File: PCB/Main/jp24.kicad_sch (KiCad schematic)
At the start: 1 part, among them U1 ORANGE_PI_CM4

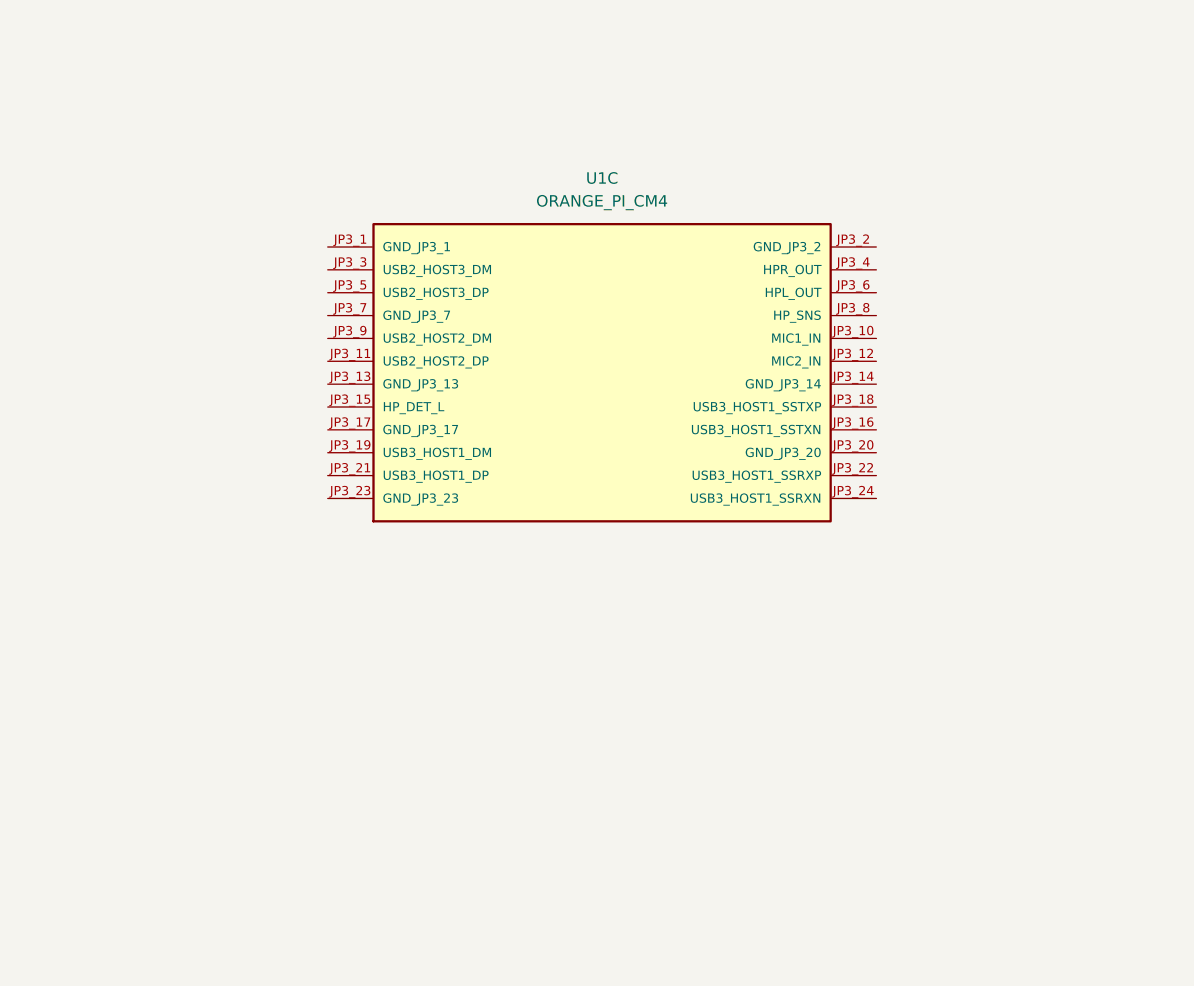
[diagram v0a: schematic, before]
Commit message: pitty
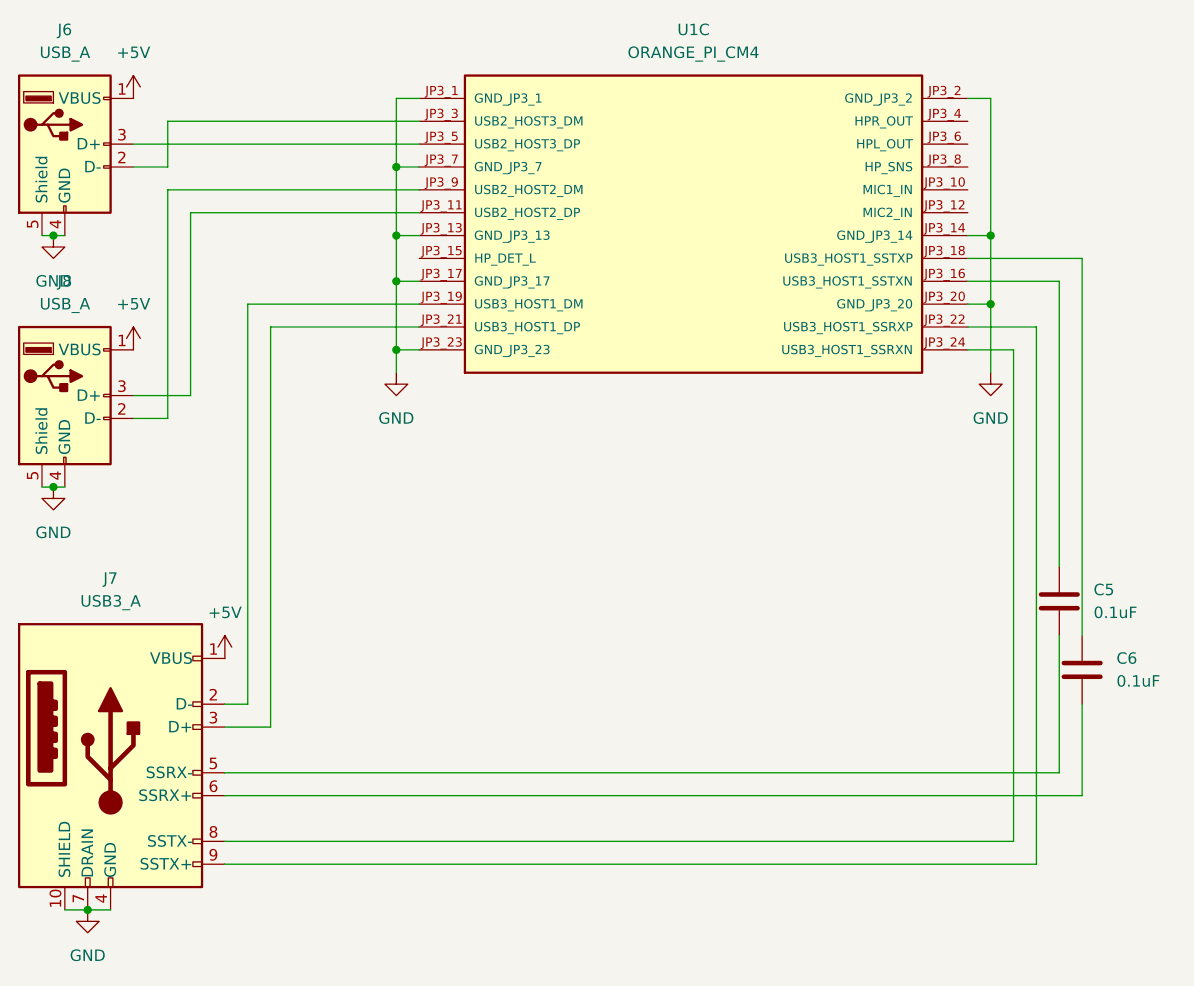
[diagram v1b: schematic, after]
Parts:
- added C5, C6: 0.1uF, symbol Device:C
- added J6, J8: USB_A, Connector_USB:USB_A_Molex_67643_Horizontal, symbol Connector:USB_A
- added J7: USB3_A, Connector_USB:USB3_A_Molex_48393-001, symbol Connector:USB3_A
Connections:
- net GND: now reaches U1.JP3_1 (GND_JP3_1)
- net GND: now also U1.JP3_13 (GND_JP3_13), U1.JP3_14 (GND_JP3_14), U1.JP3_17 (GND_JP3_17), U1.JP3_2 (GND_JP3_2), U1.JP3_20 (GND_JP3_20), U1.JP3_23 (GND_JP3_23), U1.JP3_7 (GND_JP3_7), J6.4 (GND), J6.5 (Shield), J7.10 (SHIELD), J7.4 (GND), J7.7 (DRAIN), J8.4 (GND), J8.5 (Shield)
- net at U1.JP3_11 (USB2_HOST2_DP): now also J8.3 (D+)
- net at U1.JP3_16 (USB3_HOST1_SSTXN): now also C5.1
- net at U1.JP3_18 (USB3_HOST1_SSTXP): now also C6.1
- net at U1.JP3_19 (USB3_HOST1_DM): now also J7.2 (D-)
- net at U1.JP3_21 (USB3_HOST1_DP): now also J7.3 (D+)
- net at U1.JP3_22 (USB3_HOST1_SSRXP): now also J7.9 (SSTX+)
- net at U1.JP3_24 (USB3_HOST1_SSRXN): now also J7.8 (SSTX-)
- net at U1.JP3_3 (USB2_HOST3_DM): now also J6.2 (D-)
- net at U1.JP3_5 (USB2_HOST3_DP): now also J6.3 (D+)
- net at U1.JP3_9 (USB2_HOST2_DM): now also J8.2 (D-)
- new net: C6.2, J7.6 (SSRX+)
- new net: C5.2, J7.5 (SSRX-)
- new net +5V: J6.1 (VBUS), J7.1 (VBUS), J8.1 (VBUS)
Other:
- moved on the sheet: U1C
